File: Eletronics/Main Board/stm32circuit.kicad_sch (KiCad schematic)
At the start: 6 parts, among them U3 STM32F411CEUx

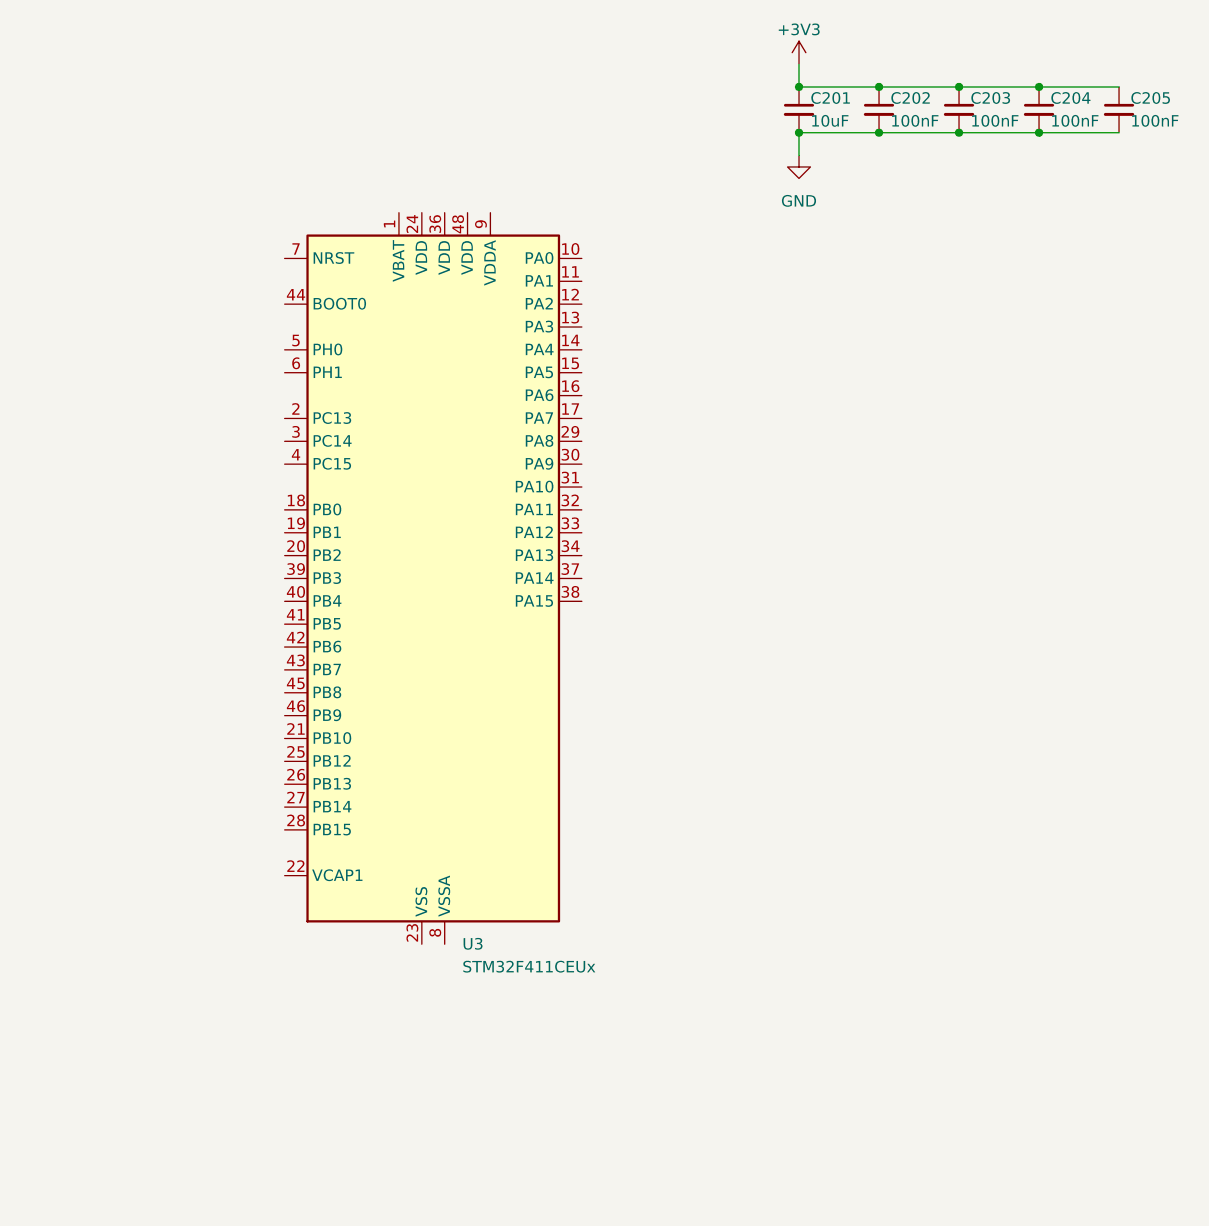
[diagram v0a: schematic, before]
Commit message: Power ok
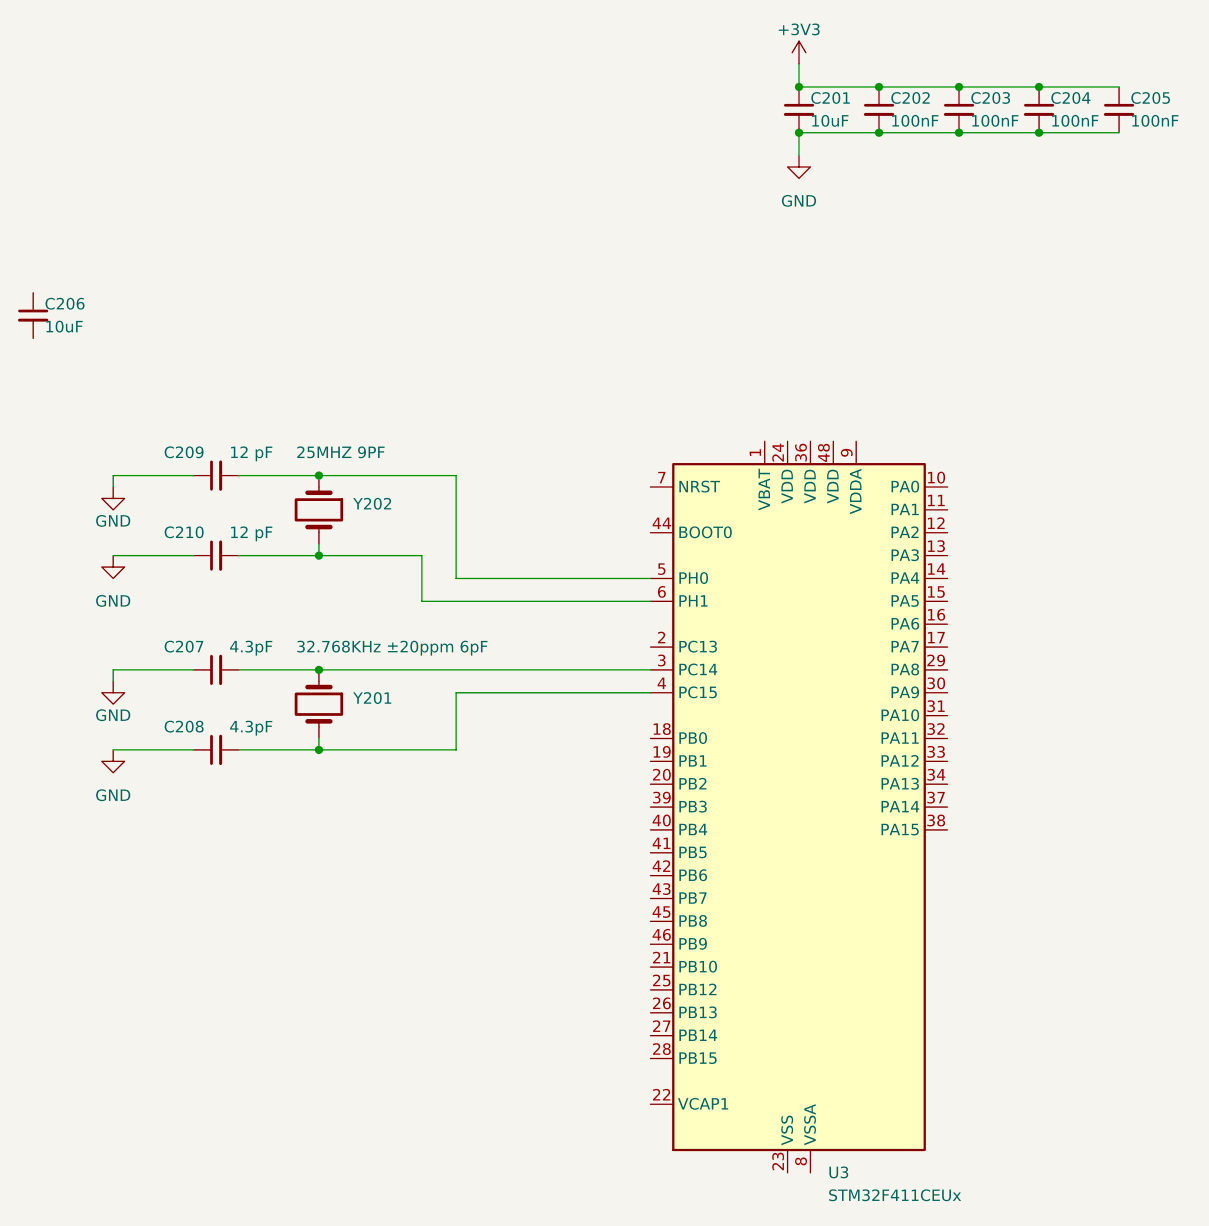
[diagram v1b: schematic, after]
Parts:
- added C206: 10uF, symbol Device:C_Small
- added C207, C208: 4.3pF, symbol Device:C_Small
- added C209, C210: 12 pF, symbol Device:C_Small
- added Y201: 32.768KHz ±20ppm 6pF, symbol Device:Crystal
- added Y202: 25MHZ 9PF, symbol Device:Crystal
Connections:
- net GND: now also C207.1, C208.1, C209.1, C210.1
- net at U3.3 (PC14): now also C207.2, Y201.1
- net at U3.4 (PC15): now also C208.2, Y201.2
- net at U3.5 (PH0): now also C209.2, Y202.1
- net at U3.6 (PH1): now also C210.2, Y202.2
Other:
- moved on the sheet: U3
